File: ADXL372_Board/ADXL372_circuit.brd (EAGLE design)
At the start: 45 x 45 mm, 57 parts, among them CN1 505568-0871, IC1 STM32L051C6, IC2 ADXL345BCCZ, IC3 ADXL372BCCZ-RL7, IC4 SI7006-A20-IM, IC6 MX25R1635FM1IL0, IC7 74AHC1G14DCK, IC8 LP5907MFX-2.5/NOPB, SW1 DHT-4235A, SW2 B3U-1000P-2P-SMD, SW3 JS202011SCQN, X1 8MHz, X2 3.2768KHZ

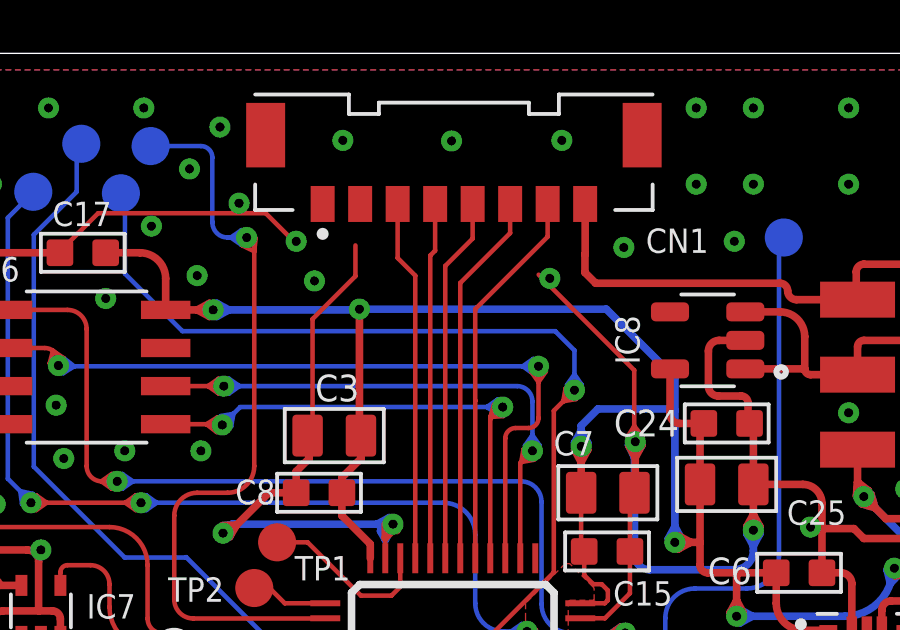
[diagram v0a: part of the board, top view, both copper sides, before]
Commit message: Update Board design
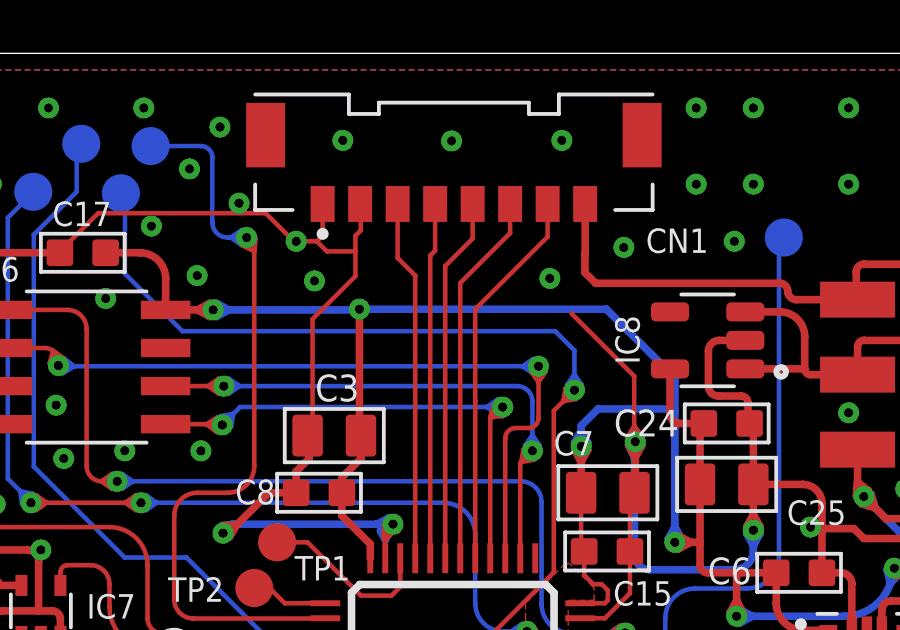
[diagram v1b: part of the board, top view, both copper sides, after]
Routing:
- net GND: track 348.4 -> 351.7 mm, vias 131 -> 134
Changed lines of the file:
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@@
 <wire x1="9.2924" y1="25.5541" x2="9.286" y2="25.566" width="0.1524" layer="1"/>
 <wire x1="11.6155" y1="22.8736" x2="11.632709375" y2="22.827684375" width="0.1524" layer="1"/>
-<wire x1="19.1209" y1="37.5742" x2="19.1209" y2="38.5992" width="0.1524" layer="1"/>
 <wire x1="17.6913" y1="36.1446" x2="19.1209" y2="37.5742" width="0.1524" layer="1"/>
 <wire x1="17.6913" y1="32.3447" x2="17.6913" y2="36.1446" width="0.1524" layer="1"/>
 <wire x1="17.6913" y1="32.3447" x2="17.526" y2="32.258" width="0.1524" layer="1"/>
-<wire x1="16.132" y1="39.6714" x2="17.0763" y2="38.7271" width="0.1524" layer="1"/>
+<wire x1="16.132" y1="39.6714" x2="17.0684" y2="38.735" width="0.1524" layer="1"/>
+<wire x1="17.0684" y1="38.735" x2="17.0763" y2="38.7271" width="0.1524" layer="1"/>
 <wire x1="10.5433" y1="39.6714" x2="16.132" y2="39.6714" width="0.1524" layer="1"/>
 <wire x1="9.2924" y1="38.4205" x2="10.5433" y2="39.6714" width="0.1524" layer="1"/>
 <wire x1="9.2924" y1="38.4205" x2="9.271" y2="38.354" width="0.1524" layer="1"/>
-<wire x1="28.4133" y1="34.4383" x2="28.4133" y2="32.578653125" width="0.1524" layer="1"/>
+<wire x1="28.4133" y1="34.2383" x2="28.4133" y2="32.578653125" width="0.1524" layer="1"/>
 <wire x1="28.4133" y1="32.578653125" x2="28.4133" y2="32.166" width="0.1524" layer="1"/>
-<wire x1="25.2282" y1="37.6234" x2="28.4133" y2="34.4383" width="0.1524" layer="1"/>
+<wire x1="26.3258" y1="36.3258" x2="28.4133" y2="34.2383" width="0.1524" layer="1"/>
 <wire x1="28.4133" y1="32.166" x2="28.448" y2="32.0548" width="0.1524" layer="1"/>
 <via x="20.3718" y="29.3068" extent="1-16" drill="0.3"/>
@@
 <vertex x="26.2636" y="27.9908"/>
 </polygon>
+<wire x1="19.1209" y1="38.9209" x2="19.3" y2="39.1" width="0.1524" layer="1"/>
+<wire x1="19.3" y1="39.1" x2="19.3" y2="39.9574" width="0.1524" layer="1"/>
+<wire x1="19.3" y1="39.9574" x2="19.2778" y2="39.9796" width="0.1524" layer="1"/>
+<wire x1="19.1209" y1="37.5742" x2="19.1209" y2="38.4" width="0.1524" layer="1"/>
+<wire x1="19.1209" y1="38.4" x2="19.1209" y2="38.9209" width="0.1524" layer="1"/>
+<wire x1="18.0278" y1="38.9278" x2="18.0278" y2="39.9796" width="0.1524" layer="1"/>
+<wire x1="17.145" y1="38.735" x2="17.0684" y2="38.735" width="0.1524" layer="1"/>
+<wire x1="17.145" y1="38.735" x2="17.835" y2="38.735" width="0.1524" layer="1"/>
+<wire x1="18.0278" y1="38.9278" x2="17.835" y2="38.735" width="0.1524" layer="1"/>
+<wire x1="17.835" y1="38.735" x2="18.17" y2="38.4" width="0.1524" layer="1"/>
+<wire x1="18.17" y1="38.4" x2="19.1209" y2="38.4" width="0.1524" layer="1"/>
+<via x="25.6" y="37.5" extent="1-16" drill="0.3"/>
+<via x="18.7" y="42.1" extent="1-16" drill="0.3"/>
+<via x="26" y="42.1" extent="1-16" drill="0.3"/>
 </signal>
 <signal name="N$1">
@@
 <wire x1="18.2836" y1="20.0706" x2="18.543465625" y2="19.916734375" width="0.1524" layer="1"/>
 </signal>
-<signal name="N$3">
-<via x="25.6" y="37.5" extent="1-16" drill="0.3"/>
-</signal>
-<signal name="N$8">
-<via x="18.7" y="42.1" extent="1-16" drill="0.3"/>
-</signal>
-<signal name="N$9">
-<via x="26" y="42.1" extent="1-16" drill="0.3"/>
-</signal>
 </signals>
